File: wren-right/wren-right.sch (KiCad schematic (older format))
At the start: 93 parts, among them J1 TRRS_Jack, SW0 Reset, U1 ProMicro

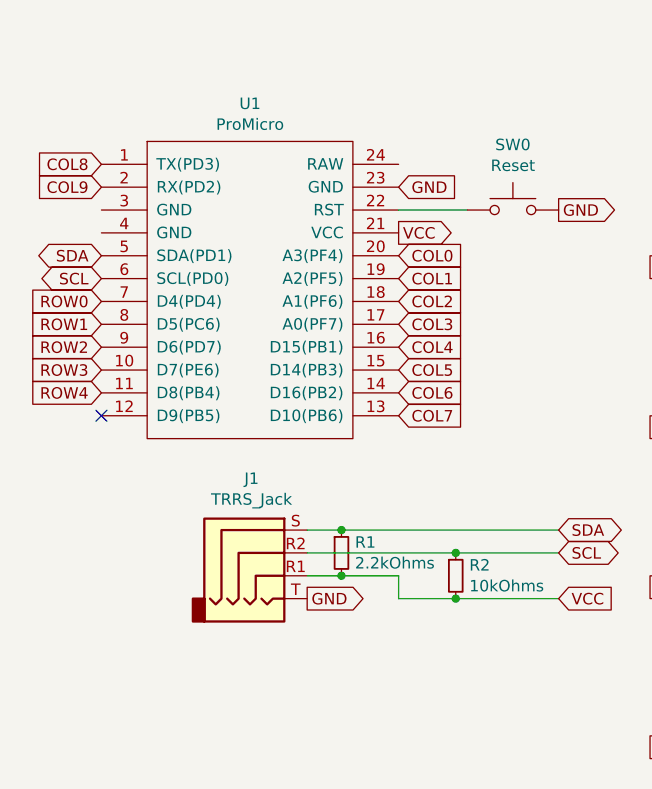
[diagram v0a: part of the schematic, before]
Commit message: Tracks Finished
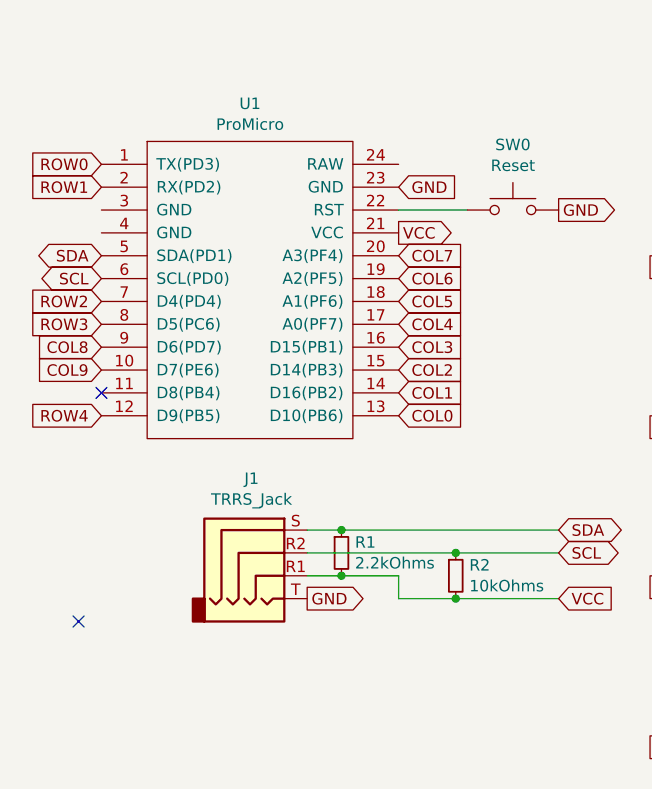
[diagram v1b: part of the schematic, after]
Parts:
- MX41: footprint MX_Only:MX-2U -> MX_Only:MX-2U-FLIPPED-ReversedStabilizers
- SW0: footprint random-keyboard-parts:SKQG-1155865 -> Button_Switch_THT:SW_PUSH_6mm
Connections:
- net COL0: now also U1.13 (D10(PB6)); no longer U1.20 (A3(PF4))
- net COL1: now also U1.14 (D16(PB2)); no longer U1.19 (A2(PF5))
- net COL2: now also U1.15 (D14(PB3)); no longer U1.18 (A1(PF6))
- net COL3: now also U1.16 (D15(PB1)); no longer U1.17 (A0(PF7))
- net COL4: now also U1.17 (A0(PF7)); no longer U1.16 (D15(PB1))
- net COL5: now also U1.18 (A1(PF6)); no longer U1.15 (D14(PB3))
- net COL6: now also U1.19 (A2(PF5)); no longer U1.14 (D16(PB2))
- net COL7: now also U1.20 (A3(PF4)); no longer U1.13 (D10(PB6))
- net COL8: now also U1.9 (D6(PD7)); no longer U1.1 (TX(PD3))
- net COL9: now also U1.10 (D7(PE6)); no longer U1.2 (RX(PD2))
- net ROW0: now also U1.1 (TX(PD3)); no longer U1.7 (D4(PD4))
- net ROW1: now also U1.2 (RX(PD2)); no longer U1.8 (D5(PC6))
- net ROW2: now also U1.7 (D4(PD4)); no longer U1.9 (D6(PD7))
- net ROW3: now also U1.8 (D5(PC6)); no longer U1.10 (D7(PE6))
- net ROW4: now also U1.12 (D9(PB5)); no longer U1.11 (D8(PB4))
- no-connect marks 1 -> 2
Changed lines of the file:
@@
 Text GLabel 1950 3150 0    50   BiDi ~ 0
-SCL
-Text GLabel 3950 4250 2    50   BiDi ~ 0
-SDA
-Text GLabel 3950 4350 2    50   BiDi ~ 0
 SCL
 Text GLabel 3250 2950 2    50   Output ~ 0
@@
 	1    0    0    -1
 $EndComp
-$Comp
-L Device:R_Small R2
-U 1 1 6072E460
-P 3500 4450
-F 0 "R2" H 3559 4496 50  0000 L CNN
-F 1 "10kOhms" H 3559 4405 50  0000 L CNN
-F 2 "Resistor_SMD:R_0805_2012Metric" H 3500 4450 50  0001 C CNN
-F 3 "~" H 3500 4450 50  0001 C CNN
-	1    3500 4450
-	1    0    0    -1
-$EndComp
 Wire Wire Line
 	2850 4450 3000 4450
@@
 F 0 "SW0" H 3750 3135 50  0000 C CNN
 F 1 "Reset" H 3750 3044 50  0000 C CNN
-F 2 "random-keyboard-parts:SKQG-1155865" H 3750 3050 50  0001 C CNN
+F 2 "Button_Switch_THT:SW_PUSH_6mm" H 3750 3050 50  0001 C CNN
 F 3 "~" H 3750 3050 50  0001 C CNN
 	1    3750 2850
@@
 F 0 "MX41" H 5133 5773 60  0000 C CNN
 F 1 "MX-NoLED" H 5133 5699 20  0000 C CNN
-F 2 "MX_Only:MX-2U" H 4475 5525 60  0001 C CNN
+F 2 "MX_Only:MX-2U-FLIPPED-ReversedStabilizers" H 4475 5525 60  0001 C CNN
 F 3 "" H 4475 5525 60  0001 C CNN
 	1    5100 5550
@@
 Text GLabel 9750 2350 1    50   Input ~ 0
 COL9
+Text GLabel 3250 3750 2    50   Input ~ 0
+COL0
+Text GLabel 3250 3650 2    50   Input ~ 0
+COL1
+Text GLabel 3250 3550 2    50   Input ~ 0
+COL2
+Text GLabel 3250 3450 2    50   Input ~ 0
+COL3
+Text GLabel 3250 3350 2    50   Input ~ 0
+COL4
+Text GLabel 3250 3250 2    50   Input ~ 0
+COL5
+Text GLabel 3250 3150 2    50   Input ~ 0
+COL6
 Text GLabel 3250 3050 2    50   Input ~ 0
-COL0
-Text GLabel 3250 3150 2    50   Input ~ 0
-COL1
-Text GLabel 3250 3250 2    50   Input ~ 0
-COL2
-Text GLabel 3250 3350 2    50   Input ~ 0
-COL3
-Text GLabel 3250 3450 2    50   Input ~ 0
-COL4
-Text GLabel 3250 3550 2    50   Input ~ 0
-COL5
-Text GLabel 3250 3650 2    50   Input ~ 0
-COL6
-Text GLabel 3250 3750 2    50   Input ~ 0
 COL7
+Text GLabel 1950 3450 0    50   Input ~ 0
+COL8
+Text GLabel 1950 3550 0    50   Input ~ 0
+COL9
 Text GLabel 1950 2650 0    50   Input ~ 0
-COL8
+ROW0
 Text GLabel 1950 2750 0    50   Input ~ 0
-COL9
+ROW1
 Text GLabel 1950 3250 0    50   Input ~ 0
-ROW0
+ROW2
 Text GLabel 1950 3350 0    50   Input ~ 0
-ROW1
-Text GLabel 1950 3450 0    50   Input ~ 0
-ROW2
-Text GLabel 1950 3550 0    50   Input ~ 0
 ROW3
-Text GLabel 1950 3650 0    50   Input ~ 0
+Text GLabel 1950 3750 0    50   Input ~ 0
 ROW4
-NoConn ~ 1950 3750
+NoConn ~ 1950 3650
+NoConn ~ 1850 4650
+$Comp
+L Device:R_Small R2
+U 1 1 6072E460
+P 3500 4450
+F 0 "R2" H 3559 4496 50  0000 L CNN
+F 1 "10kOhms" H 3559 4405 50  0000 L CNN
+F 2 "Resistor_SMD:R_0805_2012Metric" H 3500 4450 50  0001 C CNN
+F 3 "~" H 3500 4450 50  0001 C CNN
+	1    3500 4450
+	1    0    0    -1
+$EndComp
+Text GLabel 3950 4350 2    50   BiDi ~ 0
+SCL
+Text GLabel 3950 4250 2    50   BiDi ~ 0
+SDA
 $EndSCHEMATC

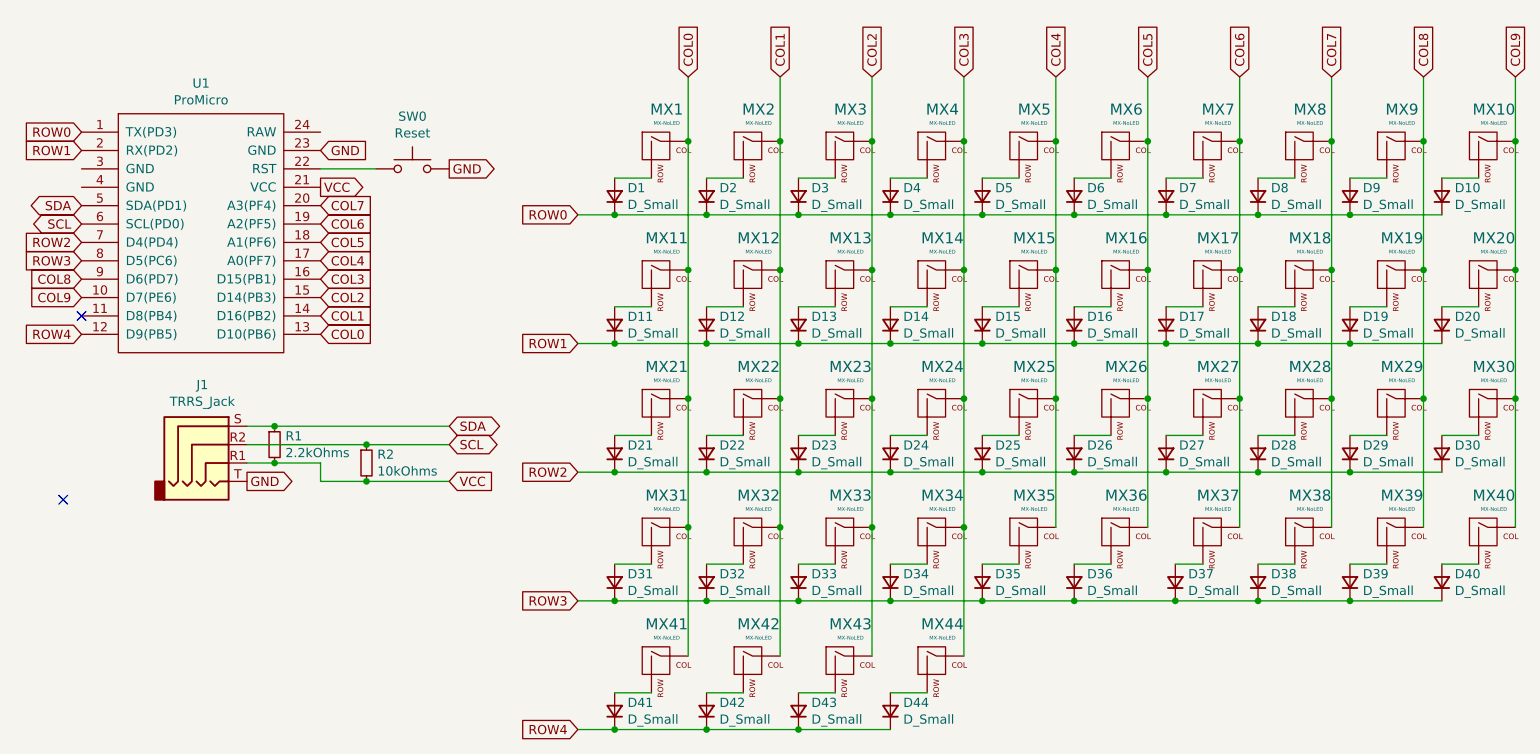
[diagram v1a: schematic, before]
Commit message: Left Side Finished
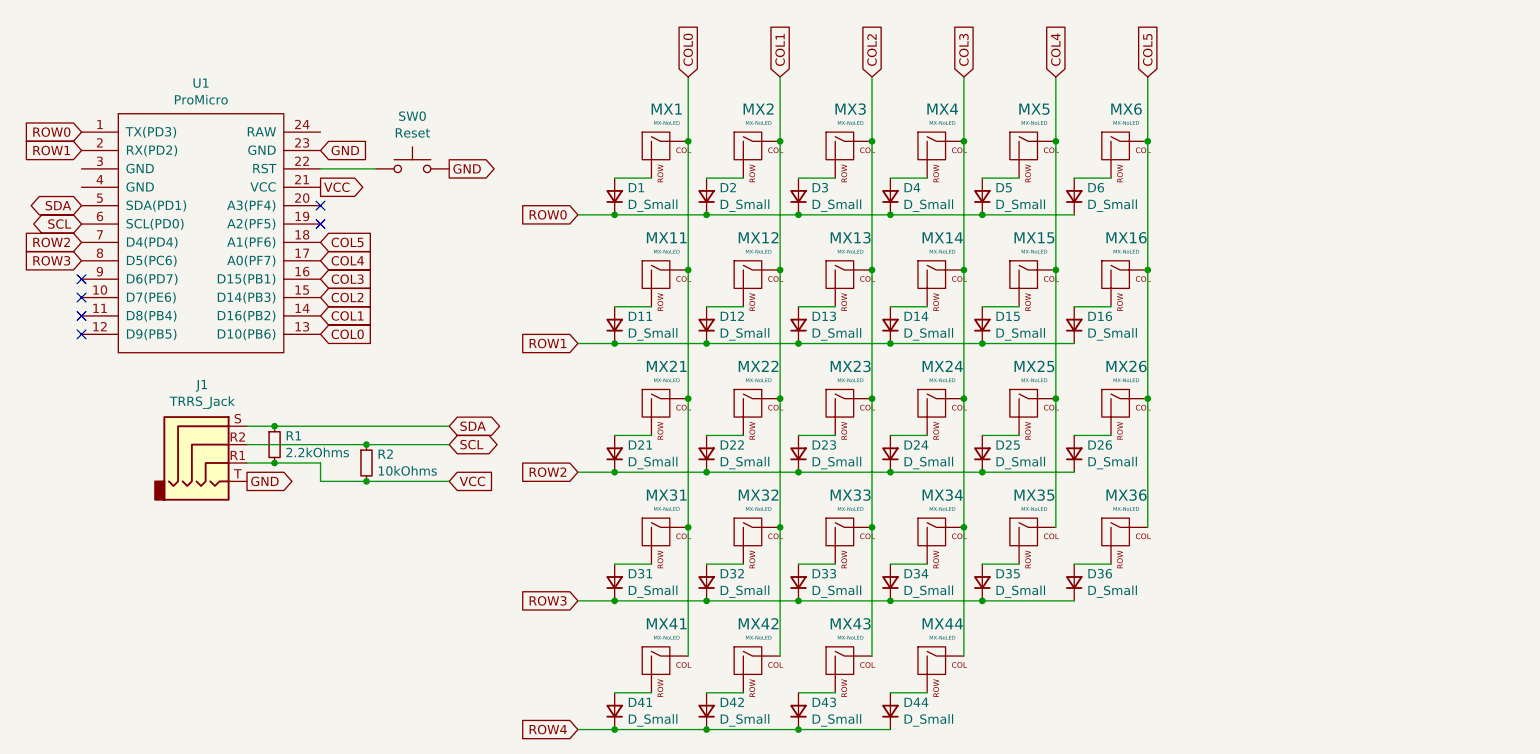
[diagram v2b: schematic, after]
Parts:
- removed D10, D17, D18, D19, D20, D27, D28, D29, D30, D37, D38, D39, D40, D7, D8, D9: D_Small, Diode_SMD:D_SOD-123, symbol Device:D_Small
- removed MX10, MX17, MX18, MX19, MX20, MX27, MX28, MX29, MX30, MX37, MX38, MX39, MX40, MX7, MX8, MX9: MX-NoLED, MX_Only:MX-1U, symbol MX_Alps_Hybrid:MX-NoLED
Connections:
- net ROW4: no longer U1.12 (D9(PB5))
- net COL6: no longer names the net of U1.19 (A2(PF5))
- net COL7: no longer names the net of U1.20 (A3(PF4))
- net COL8: no longer names the net of U1.9 (D6(PD7))
- net COL9: no longer names the net of U1.10 (D7(PE6))
- no-connect marks 2 -> 6
